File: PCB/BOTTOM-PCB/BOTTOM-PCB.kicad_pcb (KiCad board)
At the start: 4 copper layers, 40 x 40 mm, 83 parts, among them J1 12402012E212A, J2 S2B-PH-K-SLFSN, J3 Conn_01x03_Pin, J4 Conn_01x04_Pin, J5 Conn_01x04_Pin, J6 Conn_01x02_Pin, Q2 NPN, SW2 PTS810_SJM_250_SMTR_LFS, SW3 PTS810_SJM_250_SMTR_LFS, U1 ESP32-S3, U10 LP38691SD-3.3, U11 BME688, U12 RV-3028-C7_32.768KHZ_1PPM-TA-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, U13 LTR-329ALS-01, U15 MCP73832T-2ACI/MC, U16 LSM6DSO32TR, U2 MX25R6435FZAIH0, U3 DRV2605LYZFR, U4 MLX90393SLW-ABA-011-RE, U5 MAX17048G_T10, U6 TMC6300-LA-T, U8 USBLC6-2SC6, Y1 ABM12W-40.0000MHZ-8-B1U-T3

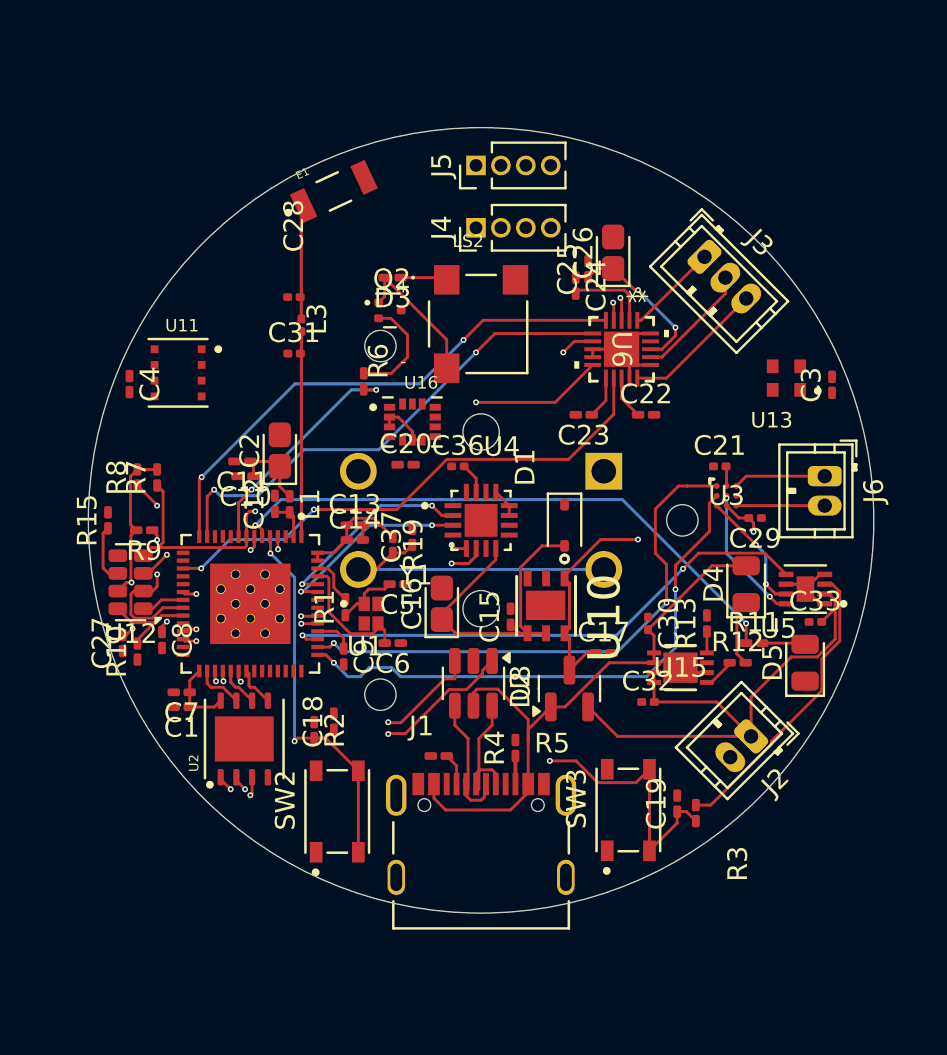
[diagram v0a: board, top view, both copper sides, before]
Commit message: I think its ready again
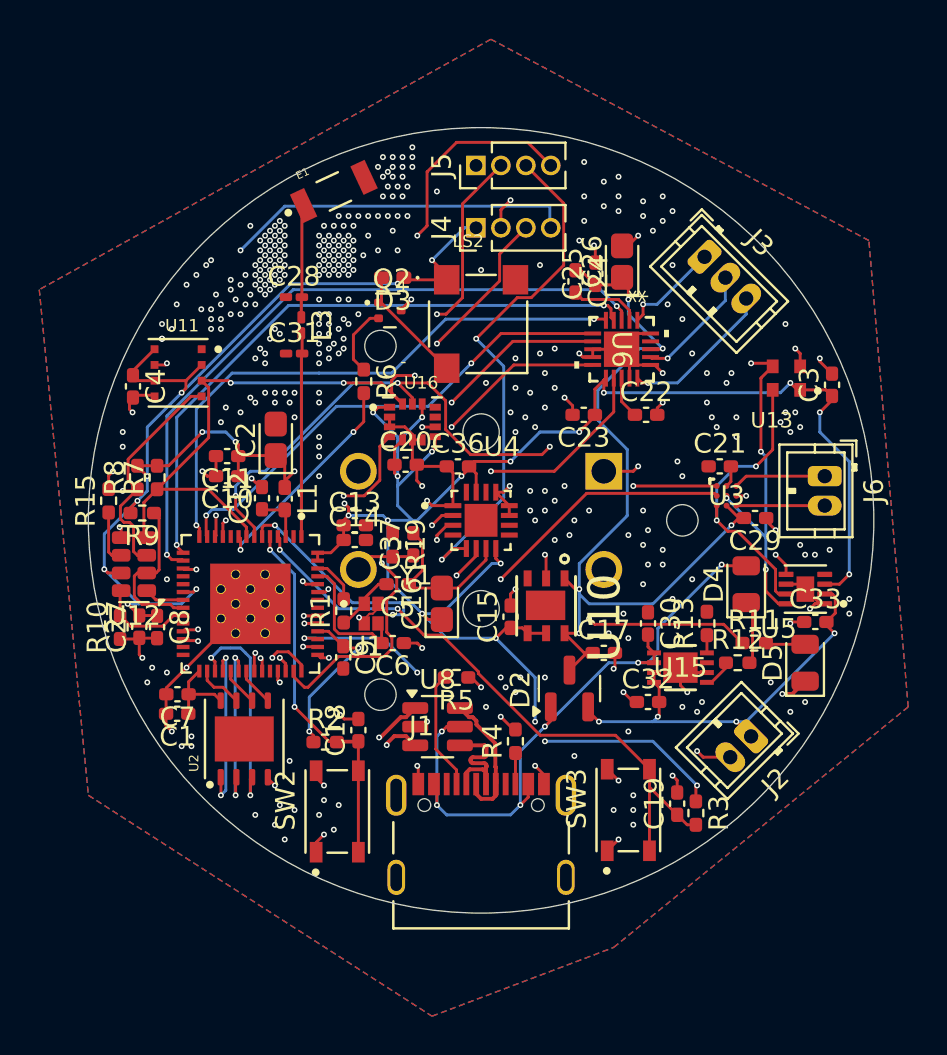
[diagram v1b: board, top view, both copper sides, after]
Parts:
- removed D1: SD03_SOD323, Diode_SMD:D_SOD-323
- C1, C10, C11, C12, C13, C14, C15, C17, C18, C19, C20, C22, C23, C24, C25, C27, C3, C37, C4, C5, C6, C7, C8, C9: footprint Capacitor_SMD:C_0201_0603Metric_Pad0.64x0.40mm_HandSolder -> Capacitor_SMD:C_0402_1005Metric_Pad0.74x0.62mm_HandSolder
- C21, C29, C30, C32, C33, C36: footprint Capacitor_SMD:C_0201_0603Metric -> Capacitor_SMD:C_0402_1005Metric_Pad0.74x0.62mm_HandSolder
- C28, C31: footprint Capacitor_SMD:C_0201_0603Metric -> Capacitor_SMD:C_0201_0603Metric_Pad0.64x0.40mm_HandSolder
- D3: footprint Diode_SMD:D_0201_0603Metric_Pad0.64x0.40mm_HandSolder -> Diode_SMD:D_0402_1005Metric_Pad0.77x0.64mm_HandSolder
- L1: footprint Inductor_SMD:L_0201_0603Metric_Pad0.64x0.40mm_HandSolder -> Inductor_SMD:L_0402_1005Metric_Pad0.77x0.64mm_HandSolder
- L3: footprint Inductor_SMD:L_0201_0603Metric -> Inductor_SMD:L_0201_0603Metric_Pad0.64x0.40mm_HandSolder
- R1, R10, R11, R12, R13, R15, R19, R2, R3, R4, R5, R6, R7, R8, R9: footprint Resistor_SMD:R_0201_0603Metric_Pad0.64x0.40mm_HandSolder -> Resistor_SMD:R_0402_1005Metric_Pad0.72x0.64mm_HandSolder
- moved R5 4.10 mm to (141.2, 92.8), turned to 180 degrees
- moved U8 2.87 mm to (140.3, 95.3), turned to 0 degrees
- moved R10 1.52 mm to (124.1, 90.2)
- moved C18 1.32 mm to (136.2, 95.4)
- moved C27 1.19 mm to (125.1, 90.2)
- moved R15 1.00 mm to (123.5, 83.8)
- moved U12 0.94 mm to (124.8, 87.0)
- moved C10 0.93 mm to (129.6, 82.5)
- moved R9 0.88 mm to (125.2, 84.4)
- moved R2 0.83 mm to (134.6, 96.0), turned to 0 degrees
- moved C11 0.82 mm to (129.6, 81.5)
- moved C12 0.72 mm to (131.3, 83.6)
- moved C8 0.71 mm to (126.0, 90.2)
- moved C26 0.64 mm to (149.7, 71.6)
- moved C2 0.59 mm to (132.0, 80.6)
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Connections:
- U1 pad 27: 21 -> unconnected-(U1-GPIO21-Pad27)
- U1 pad 36: 48 -> INT2
- U1 pad 37: 47 -> INT1
- U1 pad 38: 33 -> unconnected-(U1-GPIO33-Pad38)
- U1 pad 39: 34 -> DC
- U1 pad 40: 35 -> BACKLIGHT_EN
- U1 pad 41: 36 -> nCS
- U1 pad 42: 37 -> nRESET
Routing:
- net +3.3V: track 65.8 -> 172.3 mm, vias 4 -> 33
- net GND: track 17.4 -> 86.8 mm, vias 0 -> 356
- net nRESET: track 0.00 -> 49.3 mm, vias 0 -> 2
- net DC: track 0.00 -> 43.8 mm, vias 0 -> 2
- net nCS: track 0.00 -> 36.3 mm, vias 0 -> 1
- net UH: track 1.17 -> 34.8 mm, vias 1 -> 2
- net VH: track 0.91 -> 32.2 mm, vias 1 -> 2
- net BACKLIGHT_EN: track 0.00 -> 28.0 mm, vias 0 -> 2
- net MOSI: track 10.9 -> 35.4 mm, vias 2 -> 3
- net WL: track 1.73 -> 24.0 mm, vias 1 -> 2
- net SCL: track 47.7 -> 69.0 mm, vias 5 -> 6
- net SDA: track 46.0 -> 67.2 mm, vias 3 -> 7
- net SCLK: track 9.99 -> 29.5 mm, vias 2 -> 3
- net INT2: track 0.00 -> 19.1 mm, vias 0 -> 2
- net VL: track 6.73 -> 22.8 mm, vias 1 -> 2
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- added copper zone on B.Cu, net GND
- added copper zone on F.Cu, net GND
- added copper zone on In1.Cu, net GND
- added copper zone on In2.Cu, net GND
